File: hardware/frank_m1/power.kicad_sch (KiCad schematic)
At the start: 8 parts, among them J3 USB4215, U1 NCP1117 3.3

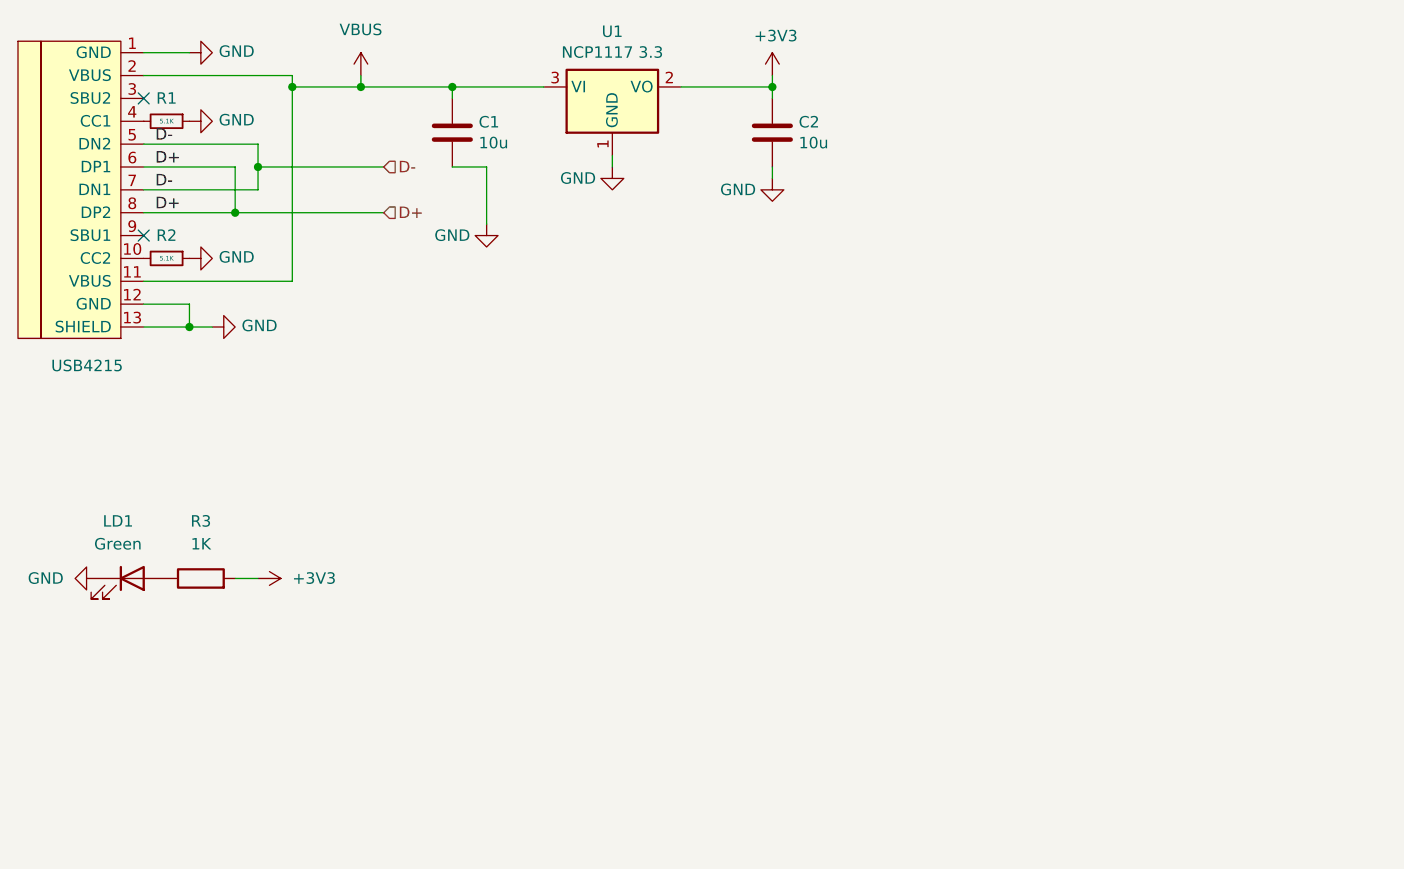
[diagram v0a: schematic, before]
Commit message: Minor updates
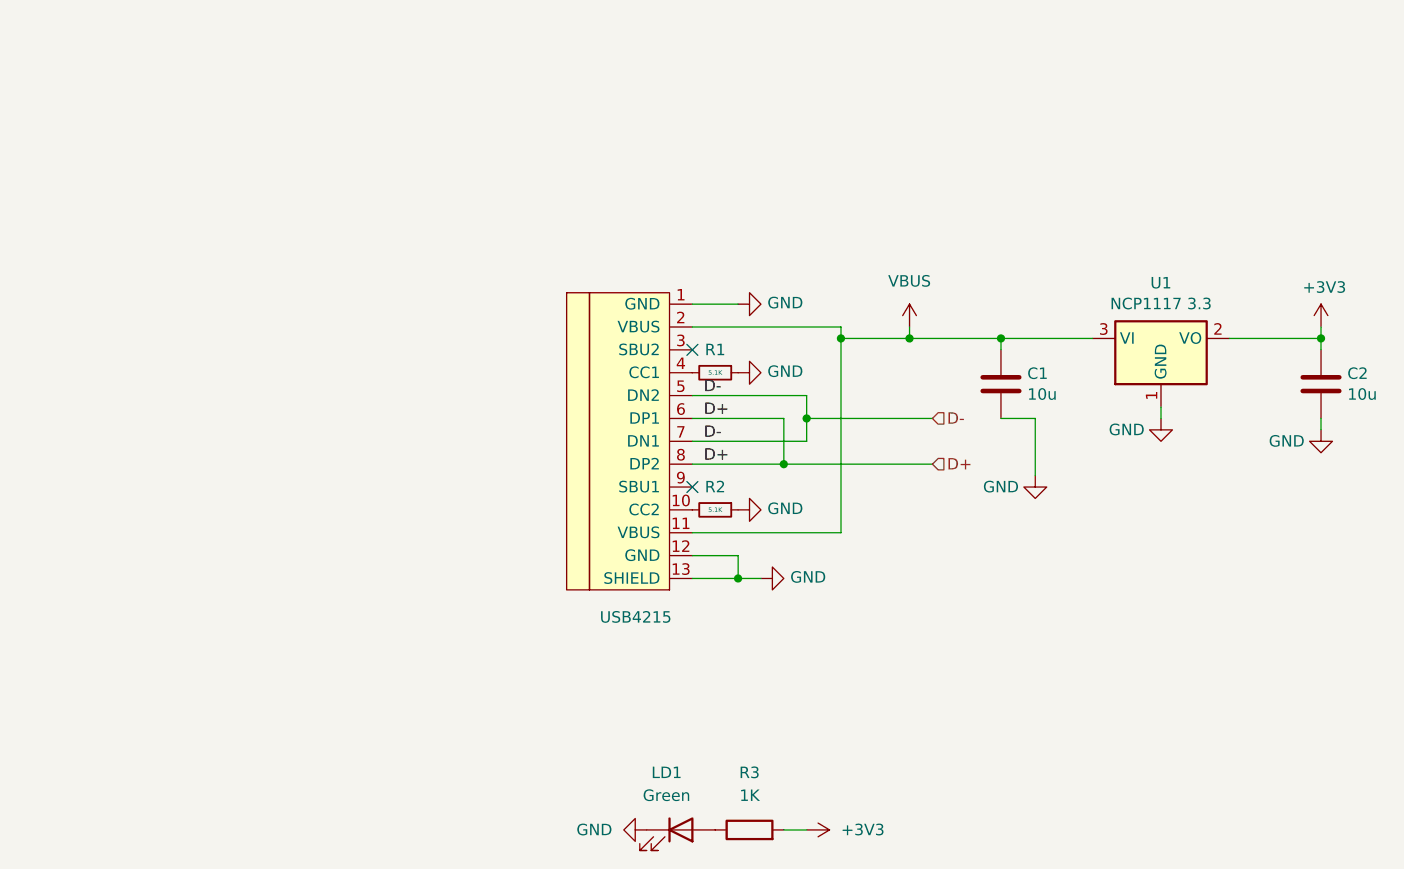
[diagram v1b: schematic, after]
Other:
- moved on the sheet: C1, C2, LD1, R1, R2, R3, U1
